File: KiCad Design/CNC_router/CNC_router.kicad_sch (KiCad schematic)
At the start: 10 parts, among them J1 Conn_01x19, J10 Conn_01x03, J2 Conn_01x19, J3 Conn_01x14, J4 Conn_01x04, J5 Conn_01x04, J6 Conn_01x04, J7 Conn_01x04, J8 Conn_01x04, J9 Conn_01x05

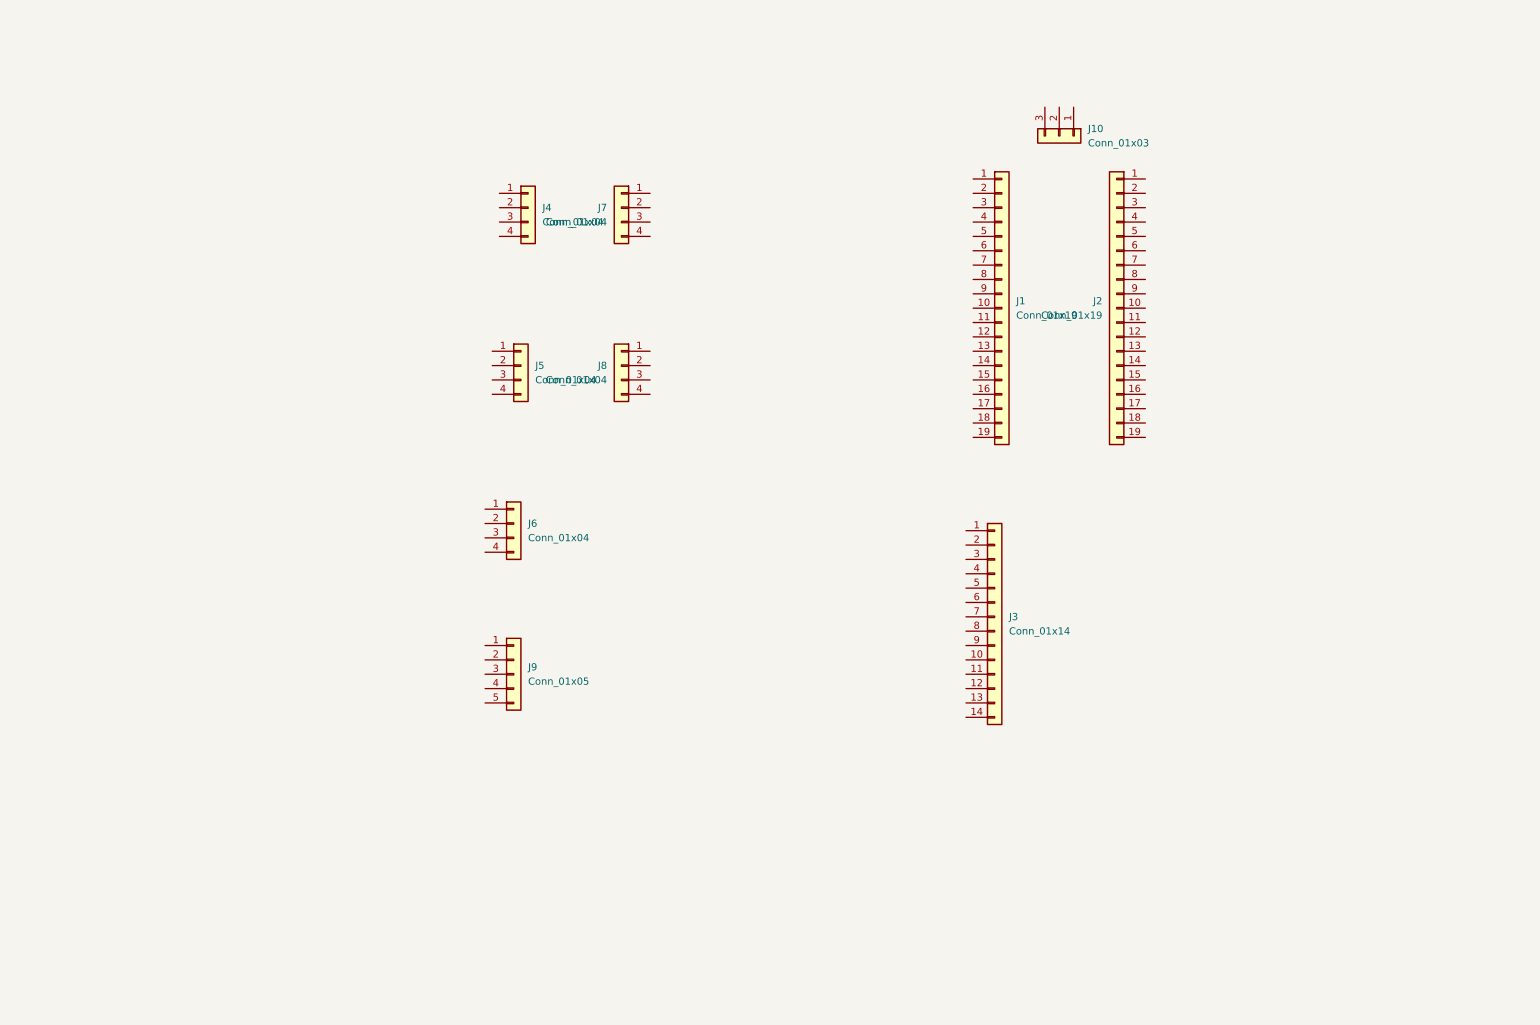
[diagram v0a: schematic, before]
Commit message: added kicad .history
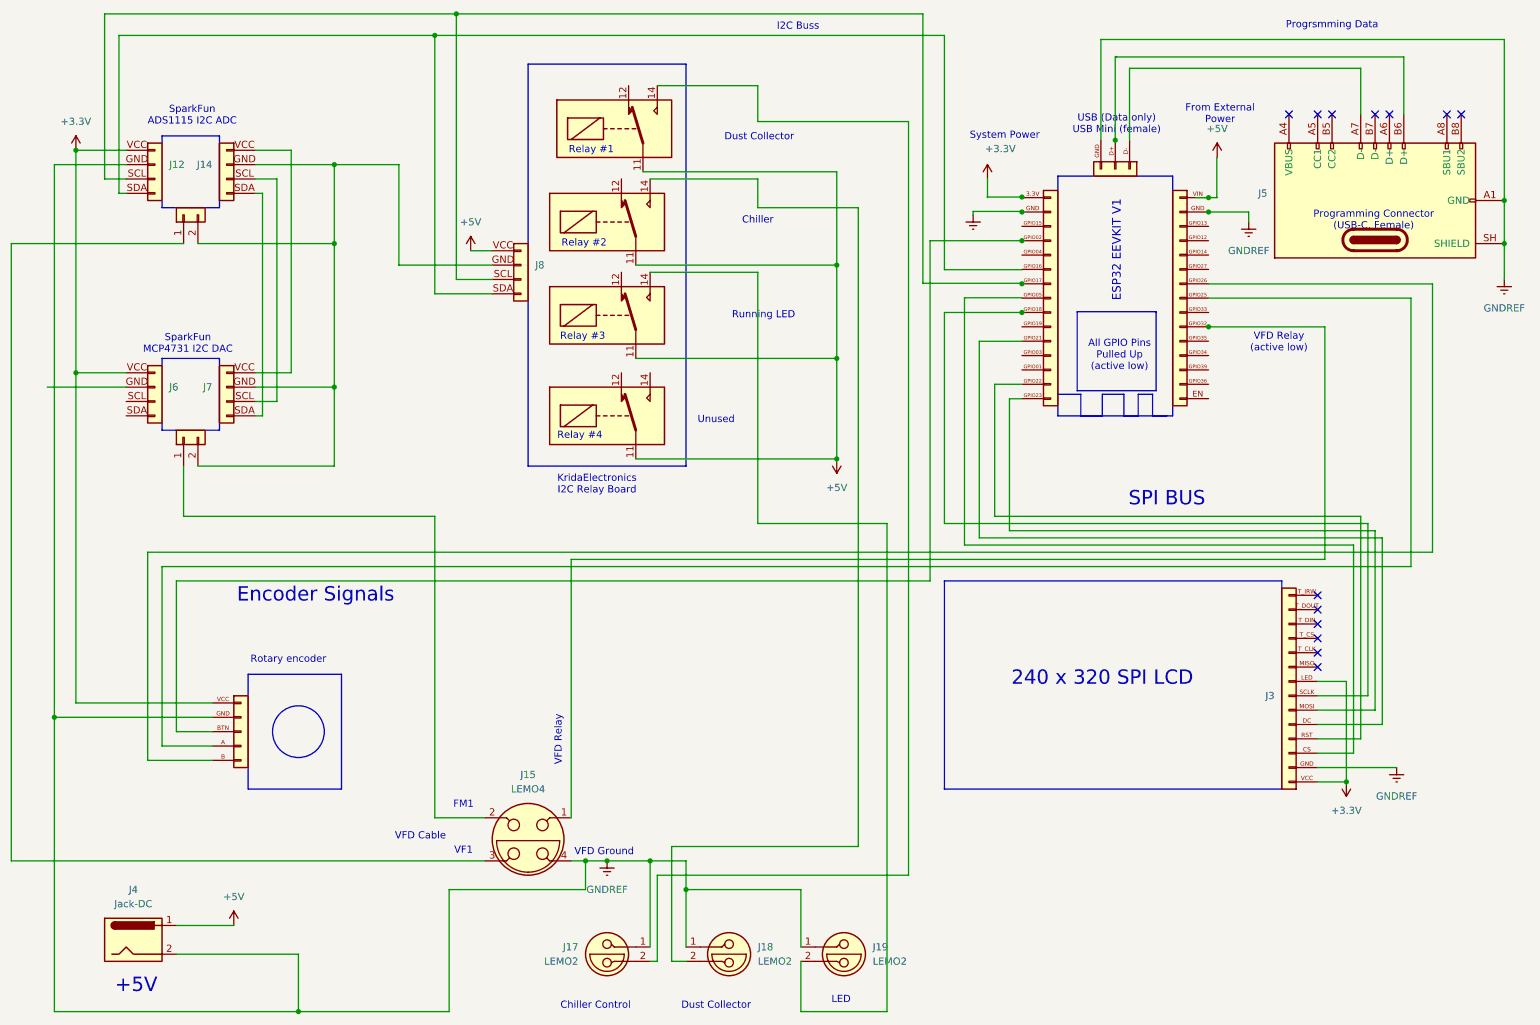
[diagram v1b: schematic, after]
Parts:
- removed J4, J5: Conn_01x04, symbol Connector_Generic:Conn_01x04
- added J11, J13: Conn_01x02, symbol Connector_Generic:Conn_01x02
- added J12, J14: Conn_01x04, symbol Connector_Generic:Conn_01x04
- added J15: LEMO4, symbol Connector:LEMO4
- added J17, J18, J19: LEMO2, symbol Connector:LEMO2
- added J4: Jack-DC, symbol Connector:Jack-DC
- added J5: USB_C_Receptacle_USB2.0_16P, symbol Connector:USB_C_Receptacle_USB2.0_16P
- added K2, K3, K4, K5: JQC-3FF-005-1Z, Relay_THT:Relay_SPDT_Hongfa_JQC-3FF_0XX-1Z, symbol Relay:JQC-3FF-005-1Z
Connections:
- new net: J11.2 (Pin_2), J13.2 (Pin_2), J14.GND (Pin_2), J7.GND (Pin_2), J8.GND (Pin_2)
- new net: J14.SCL (Pin_3), J7.SCL (Pin_3)
- new net: J14.SDA (Pin_4), J7.SDA (Pin_4)
- new net: J14.VCC (Pin_1), J7.VCC (Pin_1)
- new net: J1.GPIO17 (Pin_7), J12.SCL (Pin_3), J8.SCL (Pin_3)
- new net: J12.SDA (Pin_4), J8.SDA (Pin_4)
- new net: J13.1 (Pin_1), J15.3
- new net: J17.2, K5.14
- new net: J15.1, J2.GPIO32 (Pin_10)
- new net: J5.A4 (VBUS), J5.A9 (VBUS), J5.B4 (VBUS), J5.B9 (VBUS)
- new net: J1.GPIO02 (Pin_4), J9.BTN (Pin_3)
- new net: J19.2, K3.14
- new net: J1.GPIO18 (Pin_9), J3.SCLK (Pin_7)
- new net: J18.2, K4.14
- new net: J11.1 (Pin_1), J15.2
- new net +3.3V: J12.VCC (Pin_1), J3.LED (Pin_8), J3.VCC (Pin_1), J6.VCC (Pin_1), J9.VCC (Pin_1)
- new net +5V: J4.1, J8.VCC (Pin_1), K2.11, K3.11, K4.11, K5.11
- new net GNDREF: J1.GND (Pin_2), J12.GND (Pin_2), J15.4, J17.1, J18.1, J19.1, J3.GND (Pin_2), J4.2, J5.A1 (GND), J5.A12 (GND), J5.B1 (GND), J5.B12 (GND), J5.SH (SHIELD), J9.GND (Pin_2)
- no-connect marks 0 -> 13
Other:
- note added: "+5V"
- note added: "240 x 320 SPI LCD"
- note added: "All GPIO Pins Pulled Up (active low)"
- note added: "Chiller"
- note added: "Chiller Control"
- note added: "Dust Collector"
- note added: "ESP32 EEVKIT V1"
- note added: "Encoder Signals"
- note added: "FM1"
- note added: "From External Power"
- note added: "I2C Buss"
- note added: "KridaElectronics I2C Relay Board"
- note added: "LED"
- note added: "Programming Connector (USB-C, Female)"
- note added: "Progrsmming Data"
- note added: "Relay #1"
- note added: "Relay #2"
- note added: "Relay #3"
- note added: "Relay #4"
- note added: "Rotary encoder"
- note added: "Running LED"
- note added: "SPI BUS"
- note added: "SparkFun ADS1115 I2C ADC"
- note added: "SparkFun MCP4731 I2C DAC"
- note added: "System Power"
- note added: "USB (Data only) USB Mini (female)"
- note added: "Unused"
- note added: "VF1"
- note added: "VFD Cable"
- note added: "VFD Ground"
- note added: "VFD Relay"
- note added: "VFD Relay (active low)"
- moved on the sheet: J3
